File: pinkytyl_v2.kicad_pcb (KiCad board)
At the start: 2 copper layers, 132 x 105.9 mm, 65 parts, among them J1 50-00174, J2 Conn_01x02, J3 USB_B_Mini, J5 Conn_02x05_Odd_Even, K0 KEYSW, K10 KEYSW, K11 KEYSW, K12 KEYSW, K13 KEYSW, K14 KEYSW, K15 KEYSW, K20 KEYSW, K21 KEYSW, K22 KEYSW, K23 KEYSW, K24 KEYSW, K25 KEYSW, K30 KEYSW, K31 KEYSW, K32 KEYSW, K33 KEYSW, K34 KEYSW, K35 KEYSW, K40 KEYSW, K41 KEYSW, U1 ATmega32U4-AU, Y1 Crystal_GND24_Small

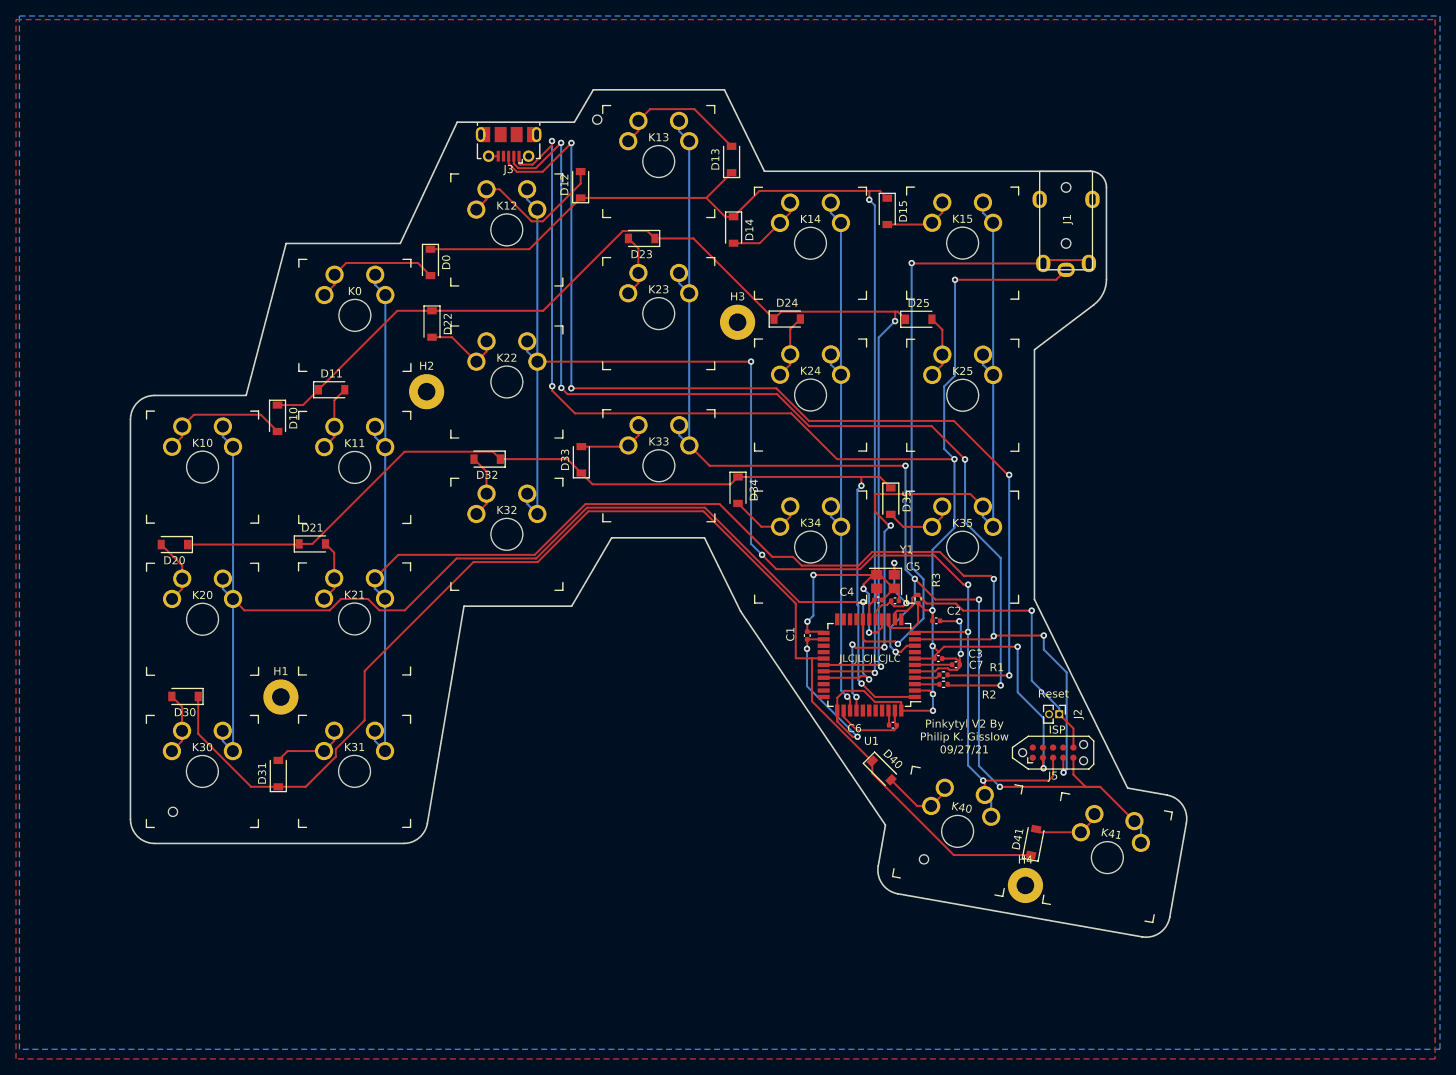
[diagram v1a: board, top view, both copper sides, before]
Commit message: Initial commit for chocs
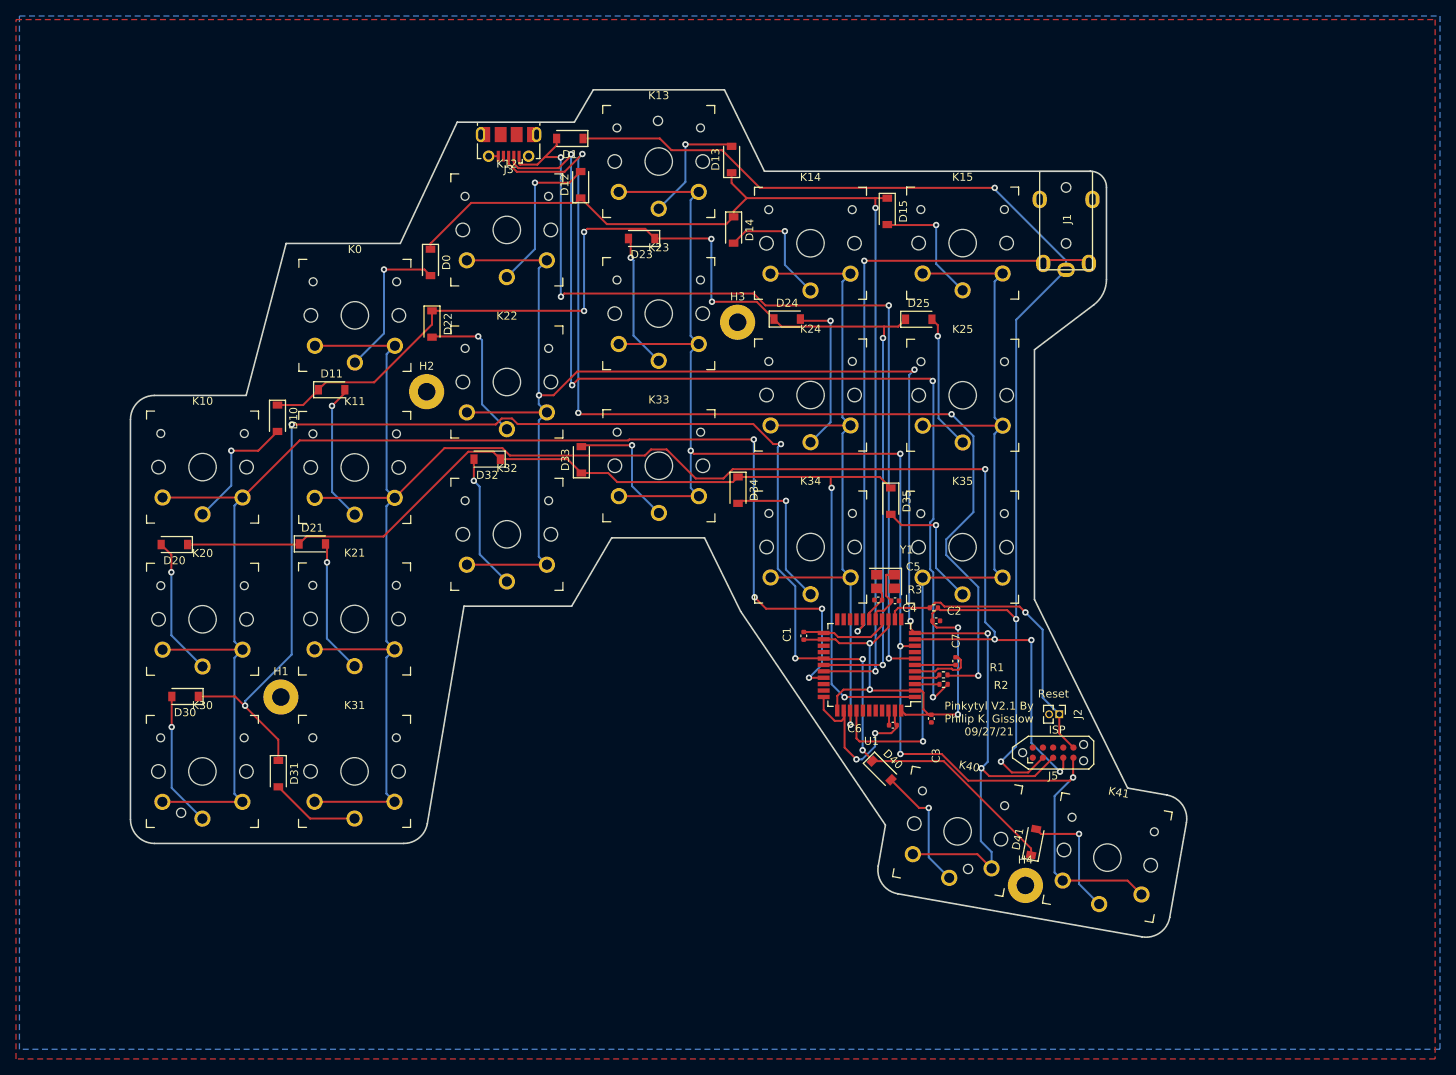
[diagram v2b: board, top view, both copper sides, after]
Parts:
- added D1: D, Diode_SMD:D_SOD-123, F.Cu at (125.5, 42.3)
- K0, K10, K11, K12, K13, K14, K15, K20, K21, K22, K23, K24, K25, K30, K31, K32, K33, K34, K35, K40, K41: footprint keyswitches:SW_MX_reversible_minimal -> keyswitches:SW_PG1350_reversible
- moved REF** 7.60 mm to (136.5, 40.1)
- moved C3 7.55 mm to (170.7, 114.8), turned to 270 degrees
- moved REF** 5.64 mm to (175.3, 133.6)
- moved R3 2.26 mm to (171.0, 100.9), turned to 0 degrees
- moved REF** 1.03 mm to (76.9, 126.5)
- moved C7 0.45 mm to (173.7, 107.6), turned to 90 degrees
- moved C1 0.44 mm to (154.7, 104.4)
- turned C4 to 180 degrees
- turned D31 to 270 degrees
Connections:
- J3 pad 1: VCC -> UVCC
- U1 pad 33: Net-(U1-Pad33) -> GND
- U1 pad 7: VCC -> UVCC
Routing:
- net UVCC: track 0.00 -> 116.1 mm, vias 0 -> 4
- net VCC: track 246.6 -> 208.6 mm, vias 12 -> 7
- net MISO: track 175.6 -> 211.8 mm
- net MOSI: track 199.6 -> 234.8 mm
- net r0: track 157.3 -> 190.0 mm, vias 0 -> 6
- net c0: track 153.9 -> 176.5 mm, vias 2 -> 4
- net GND: track 64.8 -> 42.9 mm, vias 6 -> 2
- net c3: track 164.6 -> 185.9 mm
- net c4: track 70.6 -> 89.9 mm
- net Net-(D24-Pad2): track 8.01 -> 20.1 mm, vias 0 -> 1
- net Net-(D34-Pad2): track 9.55 -> 19.1 mm, vias 0 -> 1
- net Net-(D11-Pad2): track 8.23 -> 17.4 mm, vias 0 -> 1
- net Net-(D22-Pad2): track 9.88 -> 18.9 mm, vias 0 -> 1
- net Net-(D32-Pad2): track 8.04 -> 17.0 mm, vias 0 -> 1
- net Net-(D30-Pad2): track 7.89 -> 16.9 mm, vias 0 -> 1
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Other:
- board text added: "Pinkytyl V2.1 By Philip K. Gisslow 09/27/21"
- board text removed: "JLCJLCJLCJLC"
- board text removed: "Pinkytyl V2 By Philip K. Gisslow 09/27/21"
